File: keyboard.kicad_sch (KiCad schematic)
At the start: 23 parts

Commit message: keyswitch placement
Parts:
- TP1, TP10, TP11, TP12, TP13, TP14, TP15, TP16, TP17, TP18, TP19, TP2, TP20, TP21, TP22, TP23, TP3, TP4, TP5, TP6, TP7, TP8, TP9: footprint (none) -> TestPoint:TestPoint_THTPad_D1.0mm_Drill0.5mm

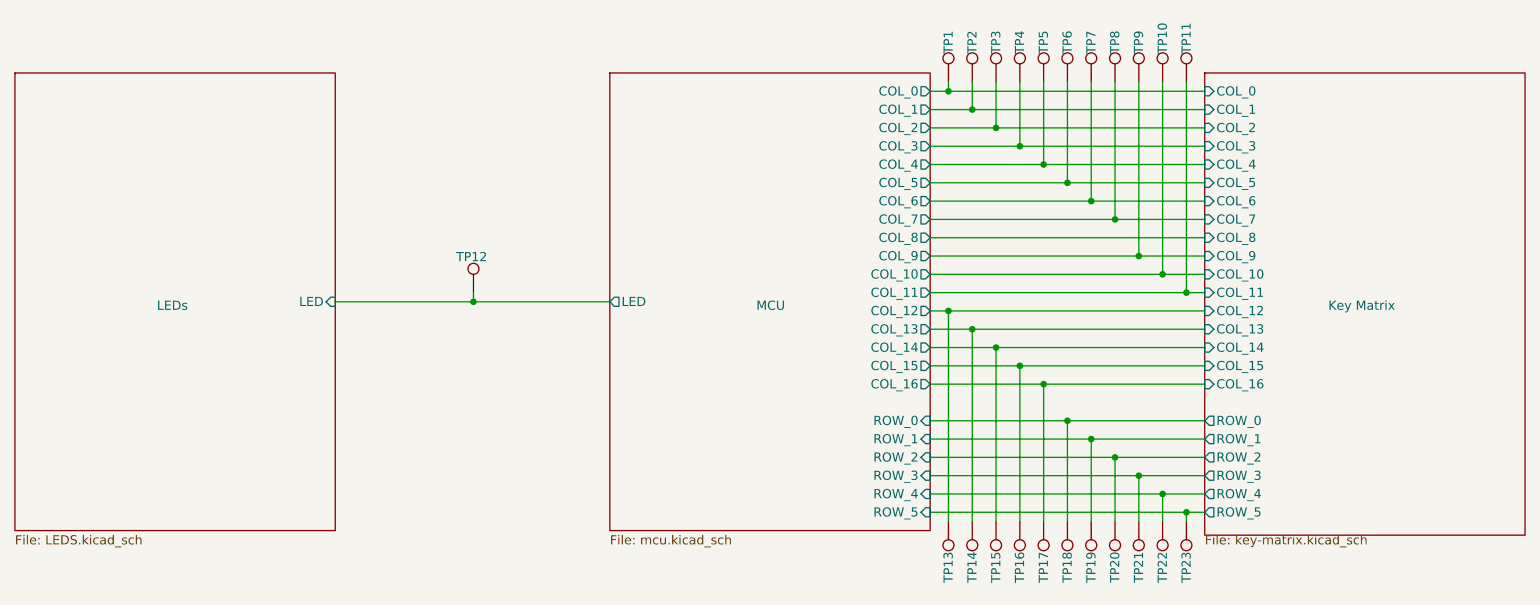
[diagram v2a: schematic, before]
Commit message: rough layout complete
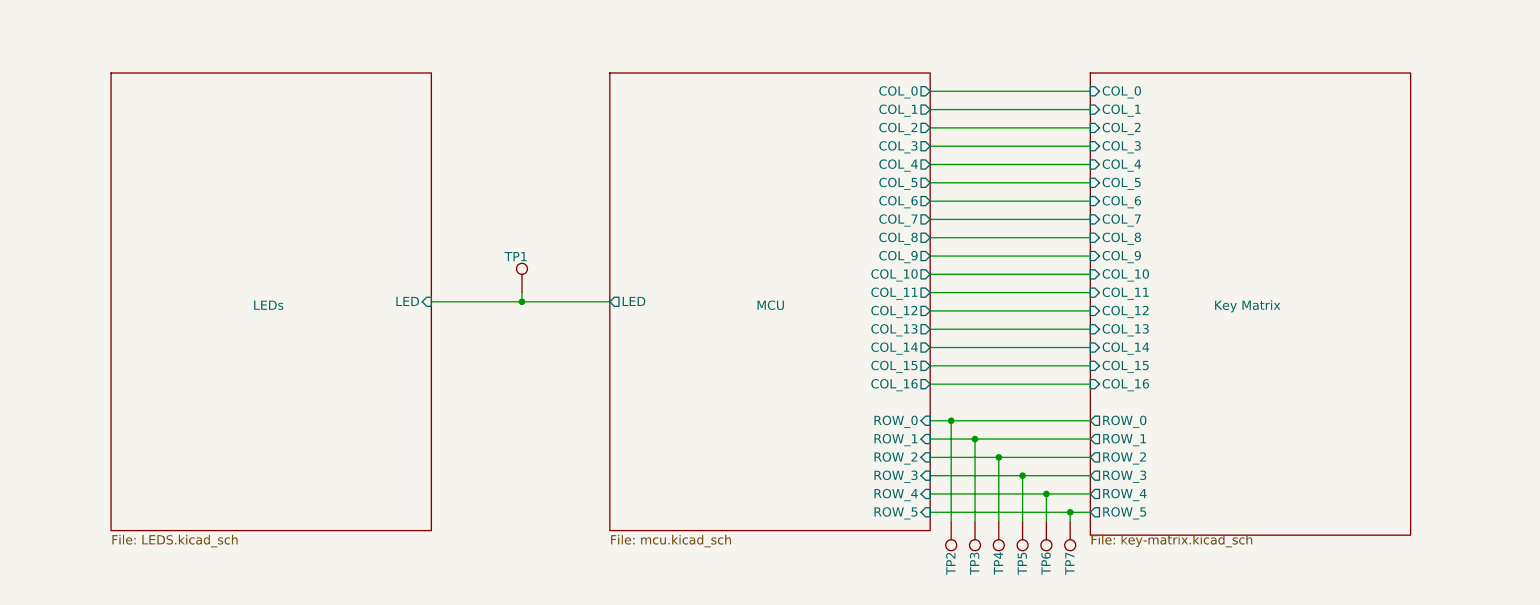
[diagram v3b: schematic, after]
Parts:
- removed TP1, TP10, TP11, TP13, TP14, TP15, TP16, TP17, TP2, TP3, TP4, TP5, TP6, TP7, TP8, TP9: TestPoint, TestPoint:TestPoint_THTPad_D1.0mm_Drill0.5mm, symbol Connector:TestPoint
- renumbered TP12 to TP1, TP18 to TP2, TP19 to TP3, TP20 to TP4, TP21 to TP5, TP22 to TP6, TP23 to TP7
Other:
- moved on the sheet: TP1, TP2, TP3, TP4, TP5, TP6, TP7
